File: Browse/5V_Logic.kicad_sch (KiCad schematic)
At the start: 13 parts, among them IC3 TPS2121RUXT

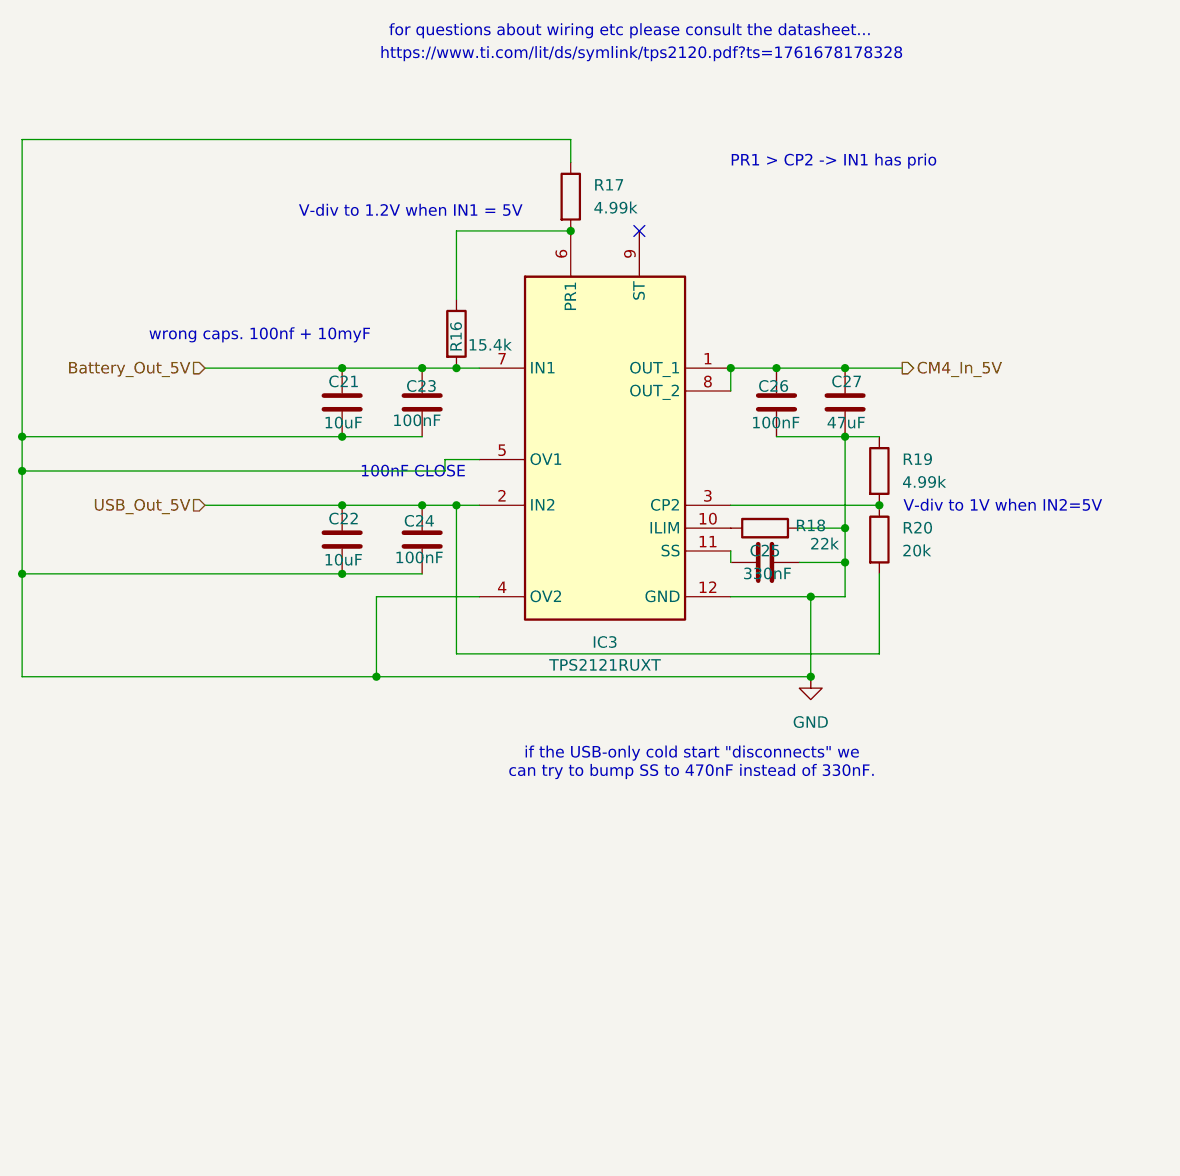
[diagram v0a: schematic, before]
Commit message: Deploying to gh-pages from @ Nautilus-UUV/nautilus-mainboard-PCB@4372544f9d98c8c318df3aa79b1ddc615587ee00 🚀
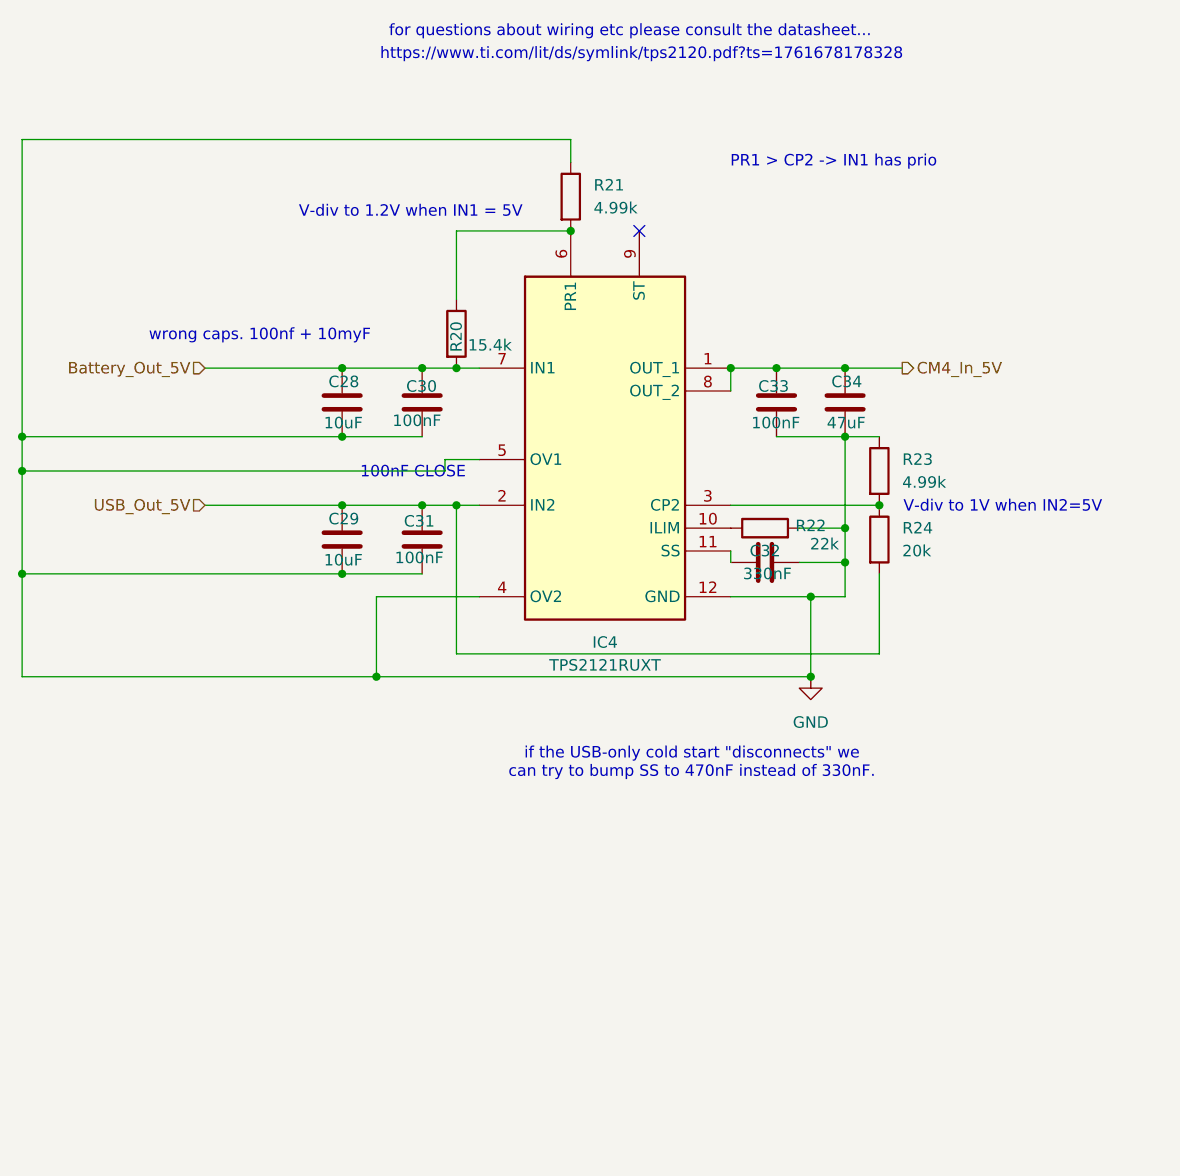
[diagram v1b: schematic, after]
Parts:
- renumbered C21 to C28, C22 to C29, C23 to C30, C24 to C31, C25 to C32, C26 to C33, C27 to C34, IC3 to IC4, R16 to R20, R17 to R21, R18 to R22, R19 to R23, R20 to R24

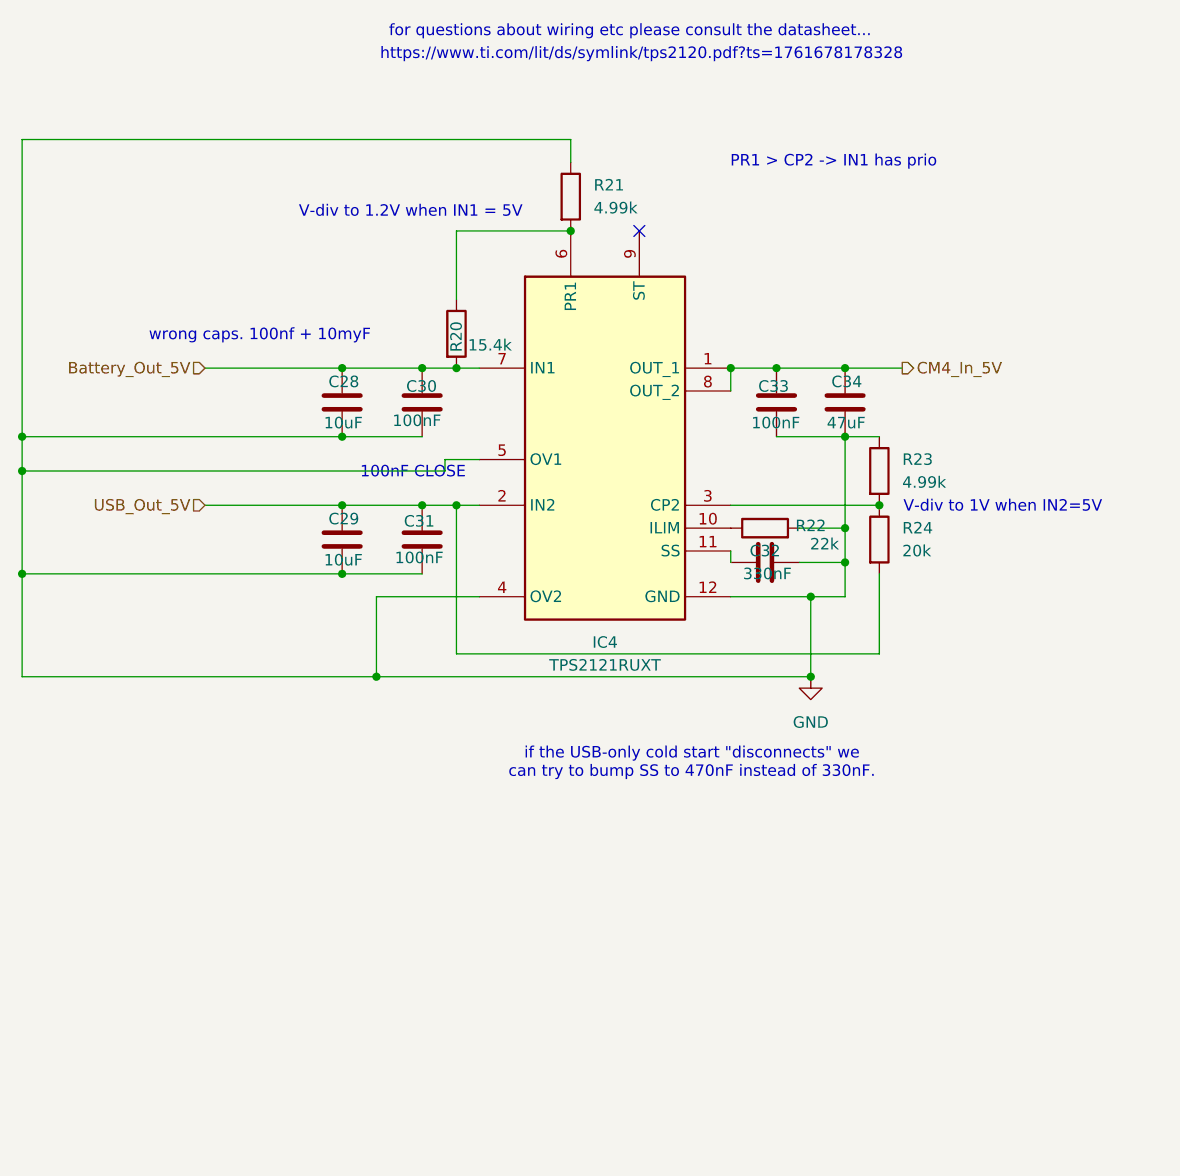
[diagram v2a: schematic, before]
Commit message: Deploying to gh-pages from @ Nautilus-UUV/nautilus-mainboard-PCB@2d3890115fd9d3c0bb909c9898aa64801bed9e67 🚀
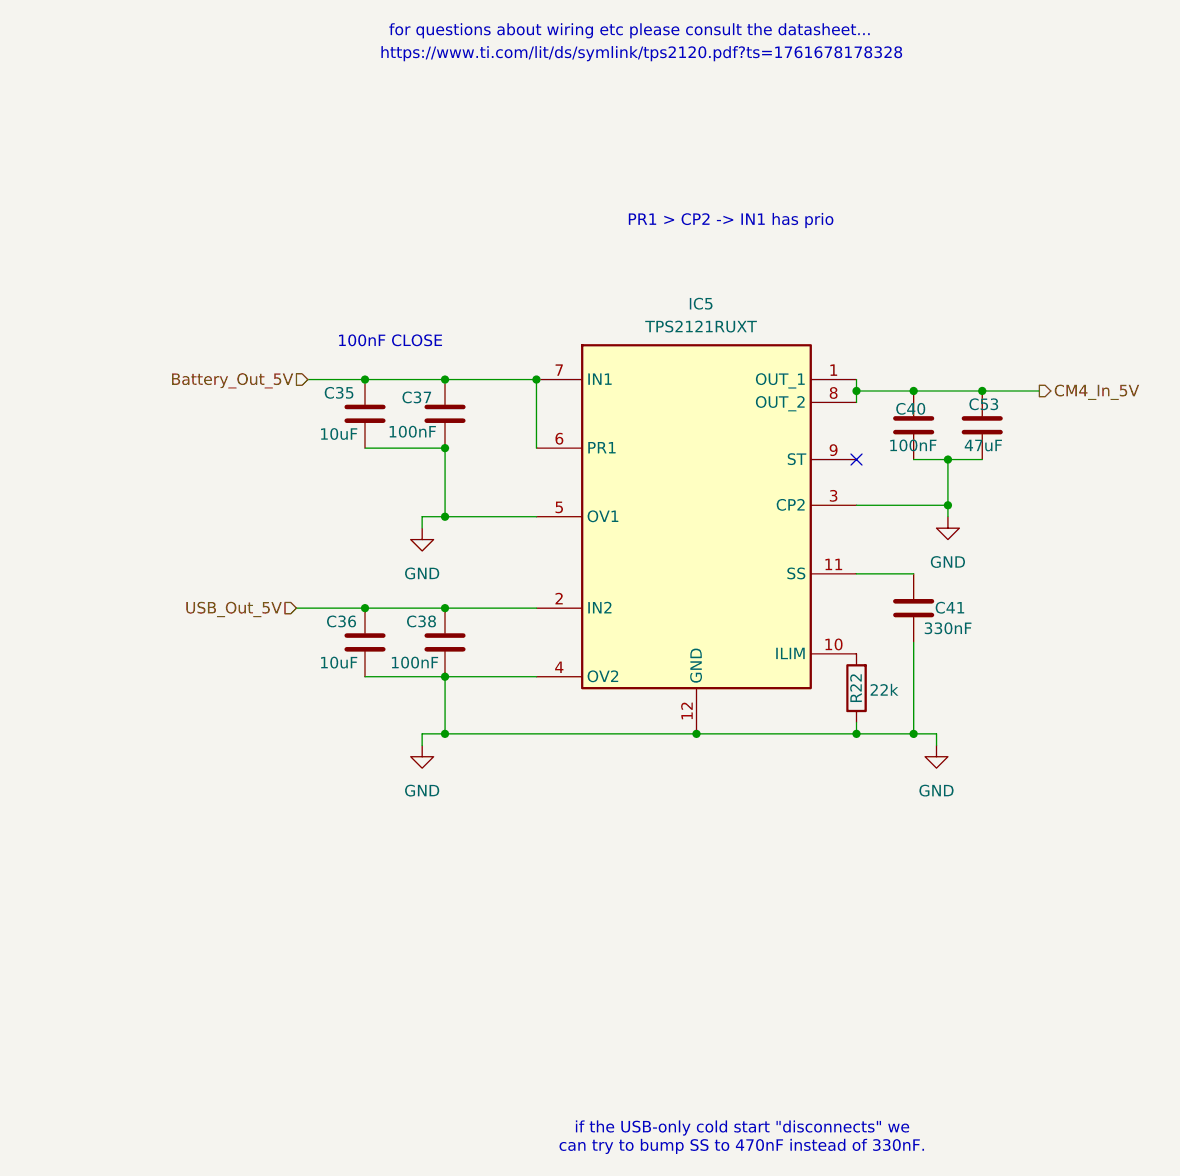
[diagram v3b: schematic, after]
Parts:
- removed C28, C29: 10uF, Capacitor_SMD:C_1210_3225Metric, symbol #dzdb:s_cap/C-MUR-GRM32EC72A106KE05
- removed C30, C31, C33: 100nF, Capacitor_SMD:C_0603_1608Metric, symbol #dzdb:g_cap/C-100n-0603
- removed C32: 330nF, Capacitor_SMD:C_0603_1608Metric, symbol #dzdb:g_cap/C-330n-0603
- removed C34: 47uF, Capacitor_SMD:C_0805_2012Metric, symbol #dzdb:s_cap/C-MUR-GRM21BR61A476ME15
- removed IC4: TPS2121RUXT, dz_dio:TI_Switchover_TPS2121RUXT, symbol #dzdb:s_misc/TEXA-595-TPS2121RUXT
- removed R20: 15.4k, Resistor_SMD:R_0603_1608Metric, symbol #dzdb:g_res/R-15.4k-0603
- removed R21, R23: 4.99k, Resistor_SMD:R_0603_1608Metric, symbol #dzdb:g_res/R-4.99k-0603
- removed R24: 20k, Resistor_SMD:R_0603_1608Metric, symbol #dzdb:g_res/R-20k-0603
- added C35, C36: 10uF, Capacitor_SMD:C_1210_3225Metric, symbol #dzdb:s_cap/C-MUR-GRM32EC72A106KE05
- added C37, C38, C40: 100nF, Capacitor_SMD:C_0603_1608Metric, symbol #dzdb:g_cap/C-100n-0603
- added C41: 330nF, Capacitor_SMD:C_0603_1608Metric, symbol #dzdb:g_cap/C-330n-0603
- added C53: 47uF, Capacitor_SMD:C_0805_2012Metric, symbol #dzdb:s_cap/C-MUR-GRM21BR61A476ME15
- added IC5: TPS2121RUXT, dz_dio:TI_Switchover_TPS2121RUXT, symbol #dzdb:s_misc/TEXA-595-TPS2121RUXT
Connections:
- net Battery_Out_5V: now also C35.1, C37.1, IC5.6 (PR1), IC5.7 (IN1)
- net CM4_In_5V: now also C40.1, C53.1, IC5.1 (OUT_1), IC5.8 (OUT_2)
- net GND: now also R22.1, C35.2, C36.2, C37.2, C38.2, C40.2, C41.1, C53.2, IC5.12 (GND), IC5.3 (CP2), IC5.4 (OV2), IC5.5 (OV1); no longer R22.2
- net USB_Out_5V: now also C36.1, C38.1, IC5.2 (IN2)
- new net: C41.2, IC5.11 (SS)
- new net: IC5.10 (ILIM), R22.2
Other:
- note removed: "V-div to 1.2V when IN1 = 5V"
- note removed: "V-div to 1V when IN2=5V"
- note removed: "wrong caps. 100nf + 10myF"
- company: (none) -> Davide
- moved on the sheet: R22
